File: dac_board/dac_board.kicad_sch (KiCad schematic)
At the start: 1 part, among them J1 AudioJack3_Ground

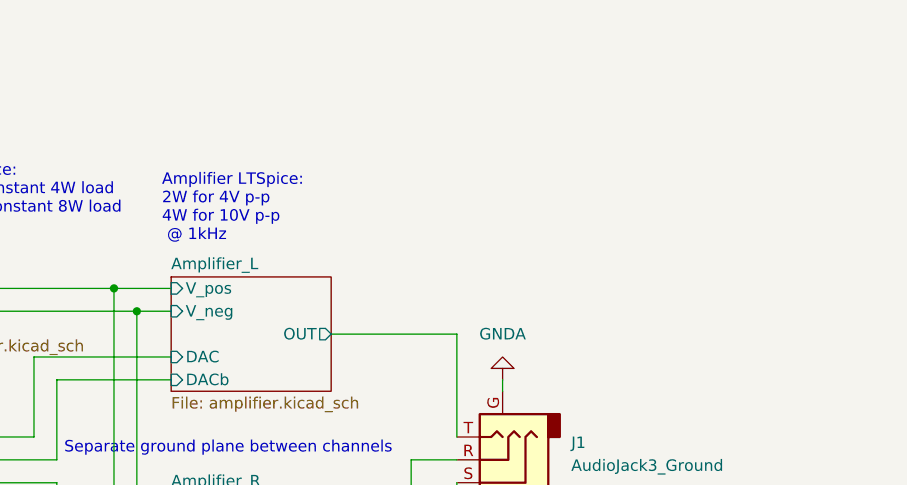
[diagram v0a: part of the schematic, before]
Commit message: Power stuff
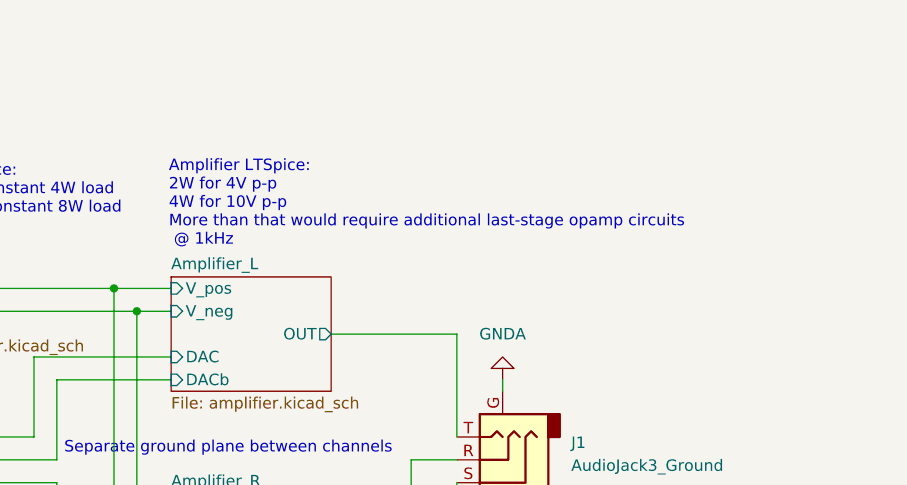
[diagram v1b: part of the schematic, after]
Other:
- note added: "Amplifier LTSpice: 2W for 4V p-p 4W for 10V p-p More than that would require additional last-stage opamp circuits @ 1kHz"
- note removed: "Amplifier LTSpice: 2W for 4V p-p 4W for 10V p-p @ 1kHz"
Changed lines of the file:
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@@
 	(generator_version "9.0")
 	(paper "A4")
-	(text "Amplifier LTSpice:\n2W for 4V p-p\n4W for 10V p-p\n @ 1kHz"
+	(text "Amplifier LTSpice:\n2W for 4V p-p\n4W for 10V p-p\nMore than that would require additional last-stage opamp circuits\n @ 1kHz"
 		(exclude_from_sim no)
-		(at 197.104 64.77 0)
+		(at 197.866 64.262 0)
 		(effects
 			(font
